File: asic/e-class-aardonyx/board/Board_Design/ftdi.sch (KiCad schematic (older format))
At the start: 62 parts, among them J1 USB_B_6PIN, J17 USB_OTG, J18 Conn_1x3_M, J2 Conn_1x8, J3 Conn_1x3_M, U1 FT2232H, U16 93LC56BT-I_OT, Y1 12MHz

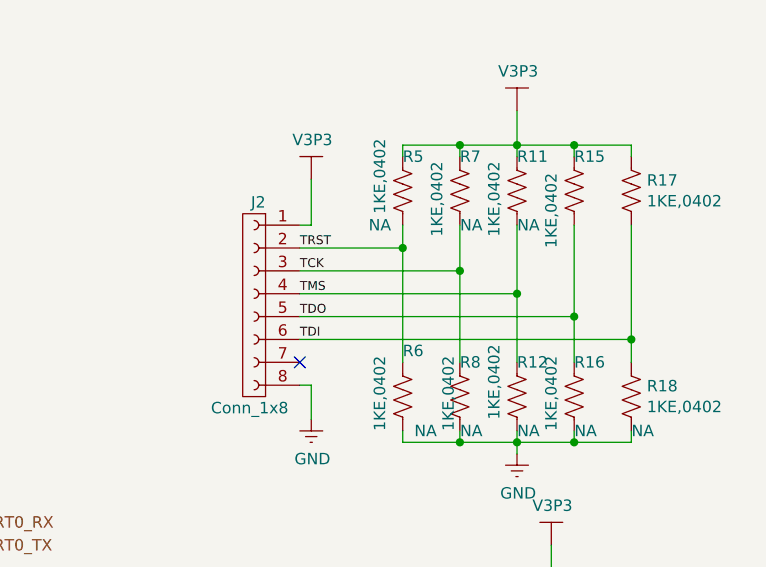
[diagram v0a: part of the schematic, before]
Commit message: Updating layout
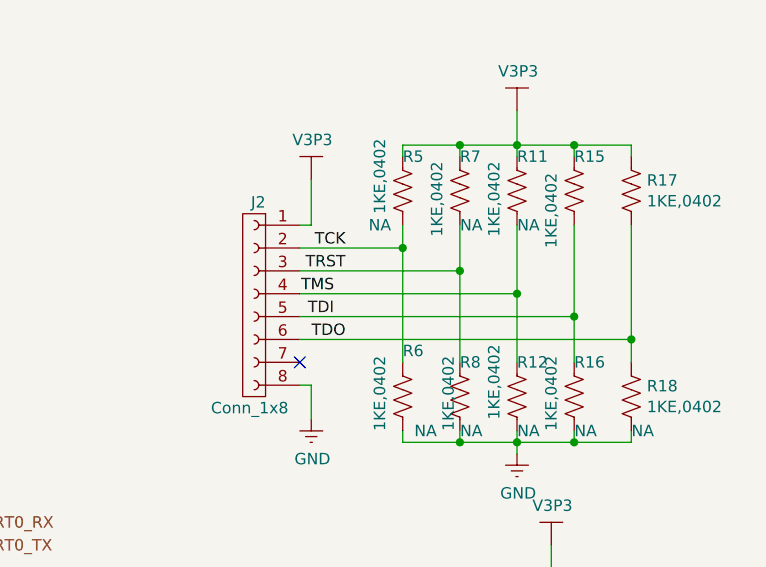
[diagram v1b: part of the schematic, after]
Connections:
- net TCK: now also J2.2 (Pin_2), R5.2, R6.1; no longer J2.3 (Pin_3), R7.2, R8.1
- net TDI: now also J2.5 (Pin_5), R15.2, R16.1; no longer J2.6 (Pin_6), R17.2, R18.1
- net TDO: now also J2.6 (Pin_6), R17.2, R18.1; no longer J2.5 (Pin_5), R15.2, R16.1
- net TRST: now also J2.3 (Pin_3), R7.2, R8.1; no longer J2.2 (Pin_2), R5.2, R6.1
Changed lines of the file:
@@
 	3800 4450 4100 4450
 Connection ~ 3800 4450
-Text Label 9300 3450 0    39   ~ 0
-TMS
-Text Label 9300 3550 0    39   ~ 0
-TDO
 $Comp
 L Aardonyx-rescue:R_US-aardonyx R5
@@
 $EndComp
 Wire Wire Line
-	9750 3250 9750 3150
-Connection ~ 9750 3250
-Wire Wire Line
-	9750 3250 9750 3750
-Wire Wire Line
-	10000 3150 10000 3350
-Connection ~ 10000 3350
-Wire Wire Line
-	10000 3350 10000 3750
-Wire Wire Line
 	9300 3650 10750 3650
 Connection ~ 10750 3650
@@
 	10500 3550 10500 3750
 Wire Wire Line
-	9300 3450 10250 3450
-Wire Wire Line
-	10250 3450 10250 3750
-Wire Wire Line
 	10500 3150 10500 3550
-Wire Wire Line
-	10250 3450 10250 3150
-Connection ~ 10250 3450
 Wire Wire Line
 	9750 2850 9750 2800
@@
 Wire Wire Line
 	9300 3550 10500 3550
-Wire Wire Line
-	9300 3350 10000 3350
-Wire Wire Line
-	9300 3250 9750 3250
 Wire Wire Line
 	6850 2650 7350 2650
@@
 Wire Wire Line
 	3300 2450 3300 2350
-Text Label 9300 3350 0    39   ~ 0
-TCK
 Text Label 4050 3750 0    50   ~ 0
 D+
@@
 Text Label 2100 3650 0    50   ~ 0
 USB_D-
-Text Label 9300 3650 0    39   ~ 0
+Wire Wire Line
+	9750 3150 9750 3250
+Wire Wire Line
+	9300 3250 9750 3250
+Connection ~ 9750 3250
+Text Label 9500 3250 2    50   ~ 0
+TCK
+Wire Wire Line
+	10000 3150 10000 3350
+Wire Wire Line
+	10000 3350 9300 3350
+Connection ~ 10000 3350
+Wire Wire Line
+	10000 3350 10000 3750
+Text Label 9500 3350 2    50   ~ 0
+TRST
+Wire Wire Line
+	9750 3250 9750 3750
+Wire Wire Line
+	10250 3150 10250 3450
+Wire Wire Line
+	9300 3450 10250 3450
+Connection ~ 10250 3450
+Wire Wire Line
+	10250 3450 10250 3750
+Text Label 9450 3450 2    50   ~ 0
+TMS
+Text Label 9450 3550 2    50   ~ 0
 TDI
-Text Label 9300 3250 0    39   ~ 0
-TRST
+Text Label 9500 3650 2    50   ~ 0
+TDO
 $EndSCHEMATC
